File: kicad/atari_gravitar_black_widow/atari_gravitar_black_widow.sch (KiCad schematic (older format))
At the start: 2 parts

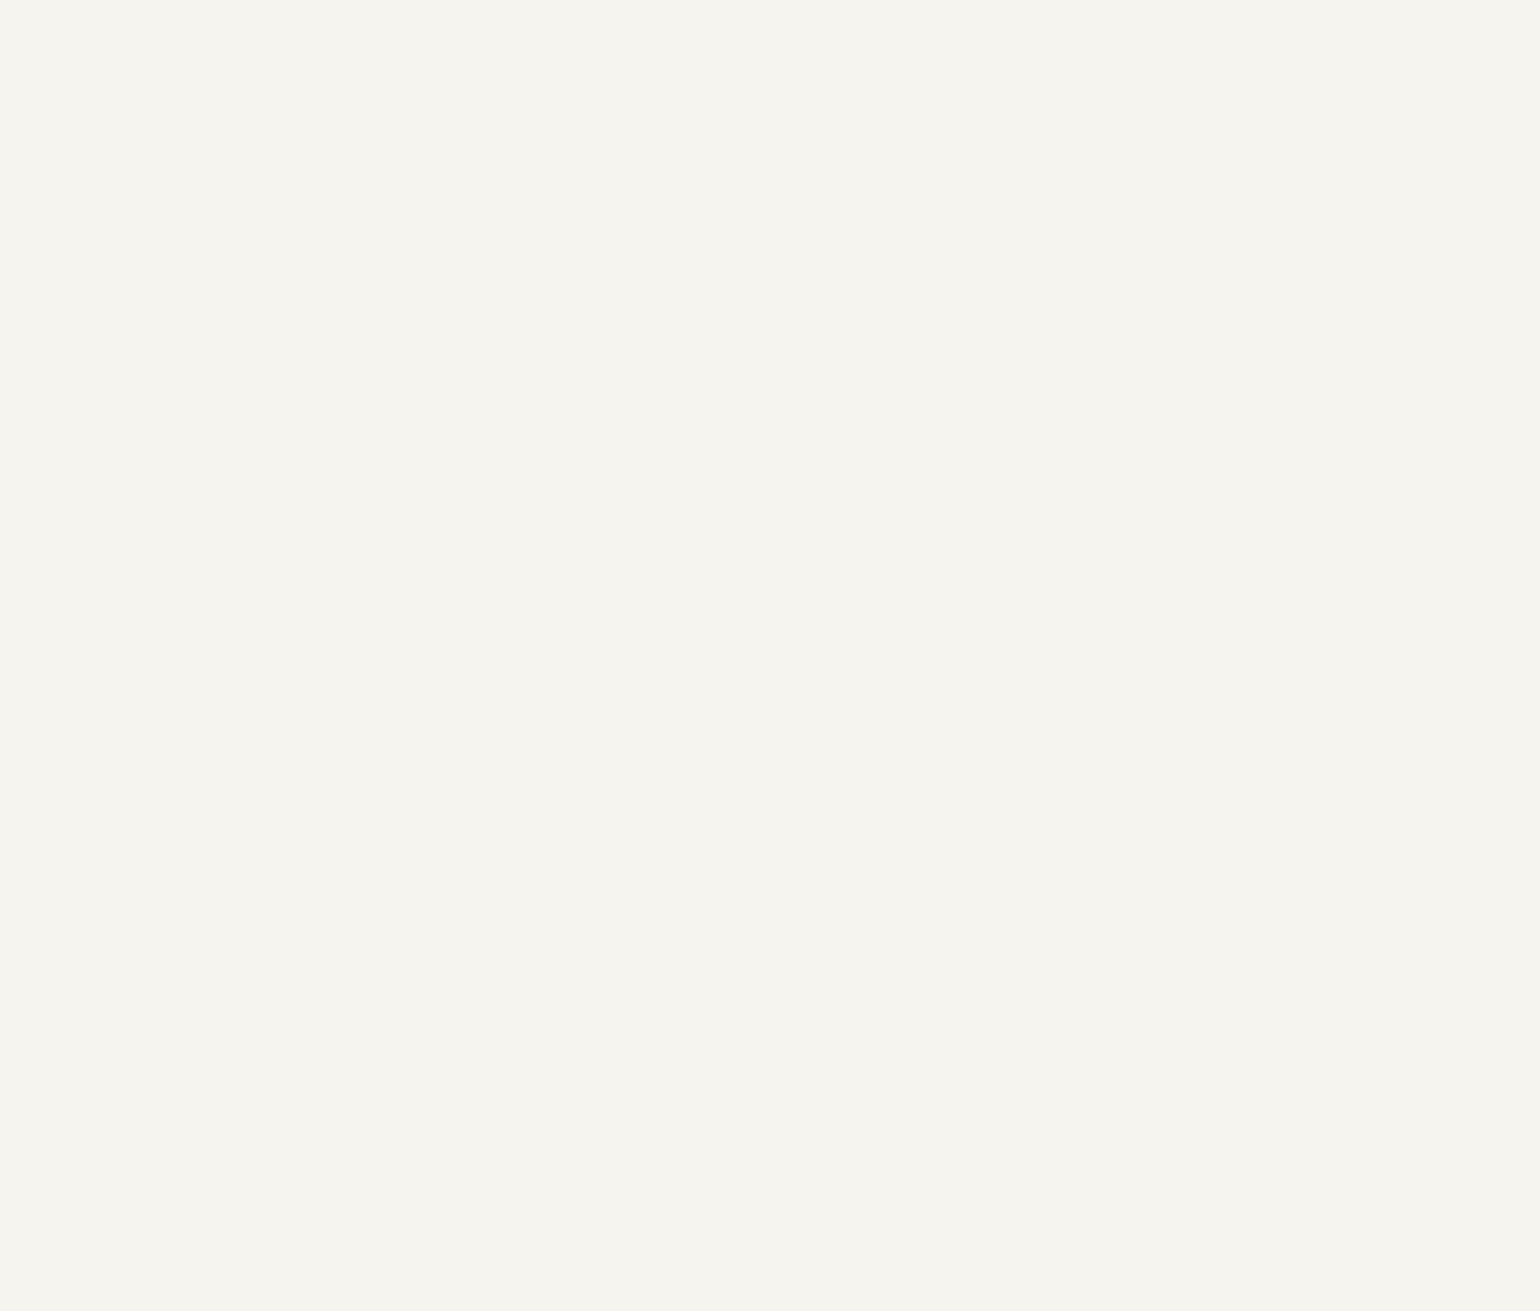
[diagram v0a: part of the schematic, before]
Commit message: First commit - AVG & VSM
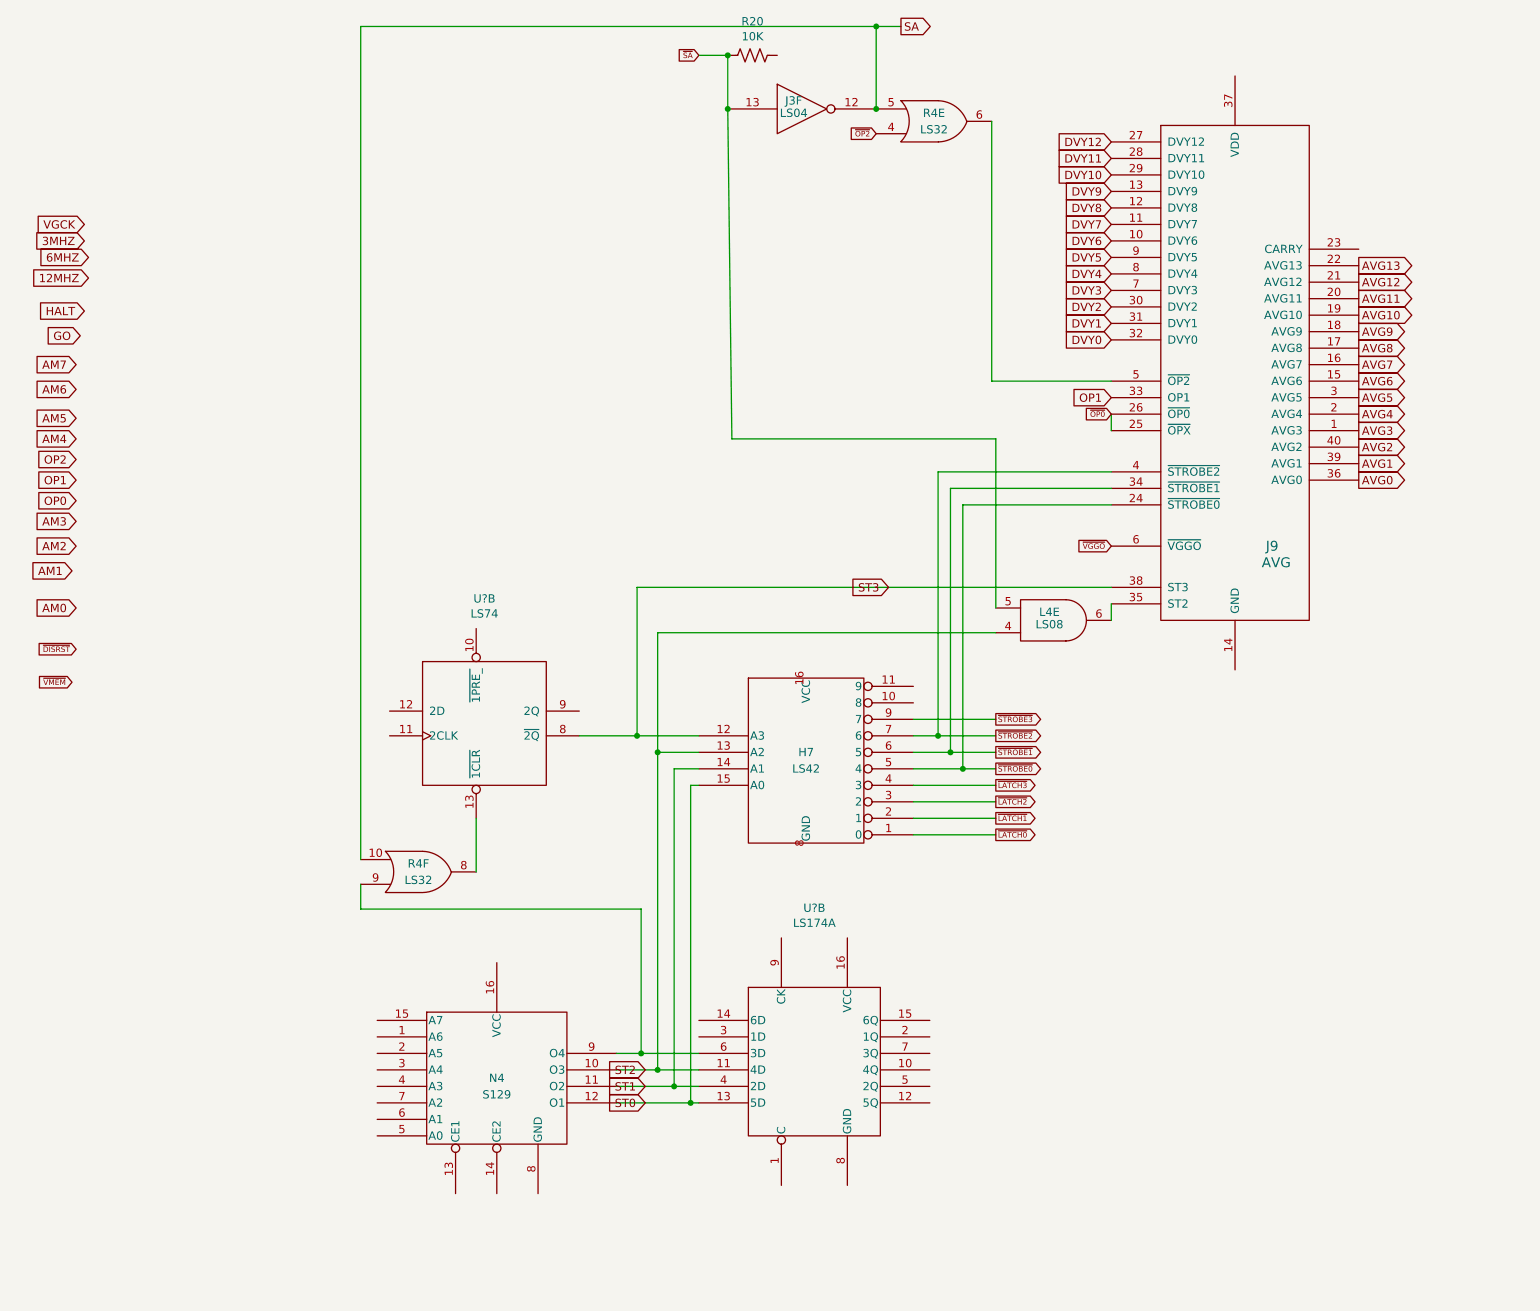
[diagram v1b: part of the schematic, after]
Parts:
- added H7: LS42, symbol Star_Wars_Vector_PCB:LS42
- added J3: LS04, symbol Star_Wars_Vector_PCB:LS04
- added J9: AVG, symbol Star_Wars_Vector_PCB:AVG
- added L4: LS08, symbol Star_Wars_Vector_PCB:LS08
- added N4: S129, symbol Star_Wars_Vector_PCB:S129
- added R20: 10K, symbol Device:R_US
- added R4: LS32, symbol Star_Wars_Vector_PCB:LS32
- added U?: LS74, symbol Star_Wars_Vector_PCB:LS74
- added U?: LS174A, symbol Star_Wars_Vector_PCB:LS174A
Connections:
- new net: J9.35 (ST2), L4.6
- new net: J9.5 (~OP2), R4.6
- new net: R4.8, U?.13 (~1CLR)
- new net: N4.9 (O4), R4.9, U?.6 (3D)
- new net AVG0: J9.36 (AVG0)
- new net AVG1: J9.39 (AVG1)
- new net AVG10: J9.19 (AVG10)
- new net AVG11: J9.20 (AVG11)
- new net AVG12: J9.21 (AVG12)
- new net AVG13: J9.22 (AVG13)
- new net AVG2: J9.40 (AVG2)
- new net AVG3: J9.1 (AVG3)
- new net AVG4: J9.2 (AVG4)
- new net AVG5: J9.3 (AVG5)
- new net AVG6: J9.15 (AVG6)
- new net AVG7: J9.16 (AVG7)
- new net AVG8: J9.17 (AVG8)
- new net AVG9: J9.18 (AVG9)
- new net DVY0: J9.32 (DVY0)
- new net DVY1: J9.31 (DVY1)
- new net DVY10: J9.29 (DVY10)
- new net DVY11: J9.28 (DVY11)
- new net DVY12: J9.27 (DVY12)
- new net DVY2: J9.30 (DVY2)
- new net DVY3: J9.7 (DVY3)
- new net DVY4: J9.8 (DVY4)
- new net DVY5: J9.9 (DVY5)
- new net DVY6: J9.10 (DVY6)
- new net DVY7: J9.11 (DVY7)
- new net DVY8: J9.12 (DVY8)
- new net DVY9: J9.13 (DVY9)
- new net OP1: J9.33 (OP1)
- new net SA: J3.12, R4.10, R4.5
- new net ST0: H7.15 (A0), N4.12 (O1), U?.13 (5D)
- new net ST1: H7.14 (A1), N4.11 (O2), U?.4 (2D)
- new net ST2: H7.13 (A2), L4.4, N4.10 (O3), U?.11 (4D)
- new net ST3: H7.12 (A3), J9.38 (ST3), U?.8 (~2Q)
- new net ~LATCH0: H7.1 (0)
- new net ~LATCH1: H7.2 (1)
- new net ~LATCH2: H7.3 (2)
- new net ~LATCH3: H7.4 (3)
- new net ~OP0: J9.25 (~OPX), J9.26 (~OP0)
- new net ~OP2: R4.4
- new net ~SA: J3.13, L4.5, R20.2
- new net ~STROBE0: H7.5 (4), J9.24 (~STROBE0)
- new net ~STROBE1: H7.6 (5), J9.34 (~STROBE1)
- new net ~STROBE2: H7.7 (6), J9.4 (~STROBE2)
- new net ~STROBE3: H7.9 (7)
- new net ~VGGO: J9.6 (~VGGO)

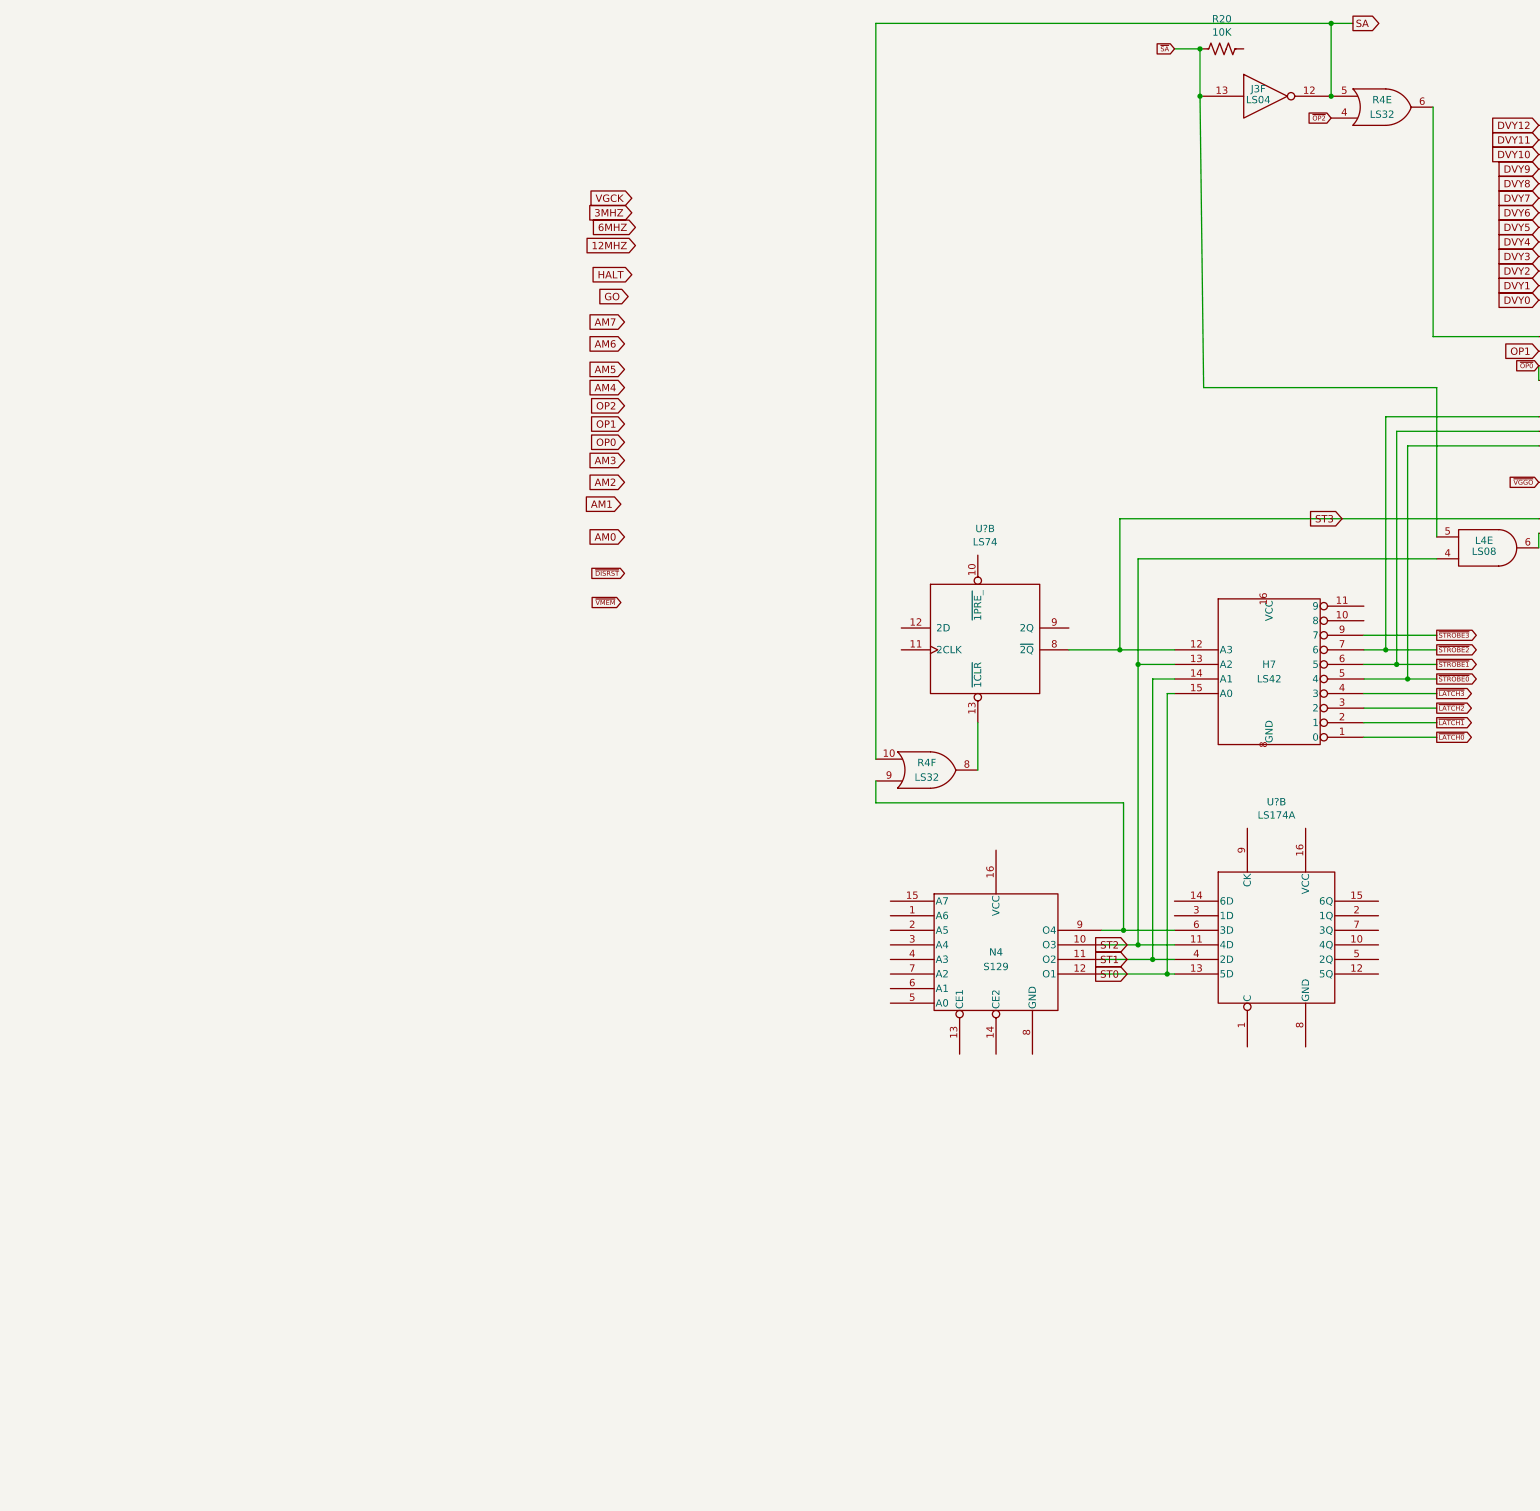
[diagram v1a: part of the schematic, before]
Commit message: 6B
More sheet 6B (but not all)
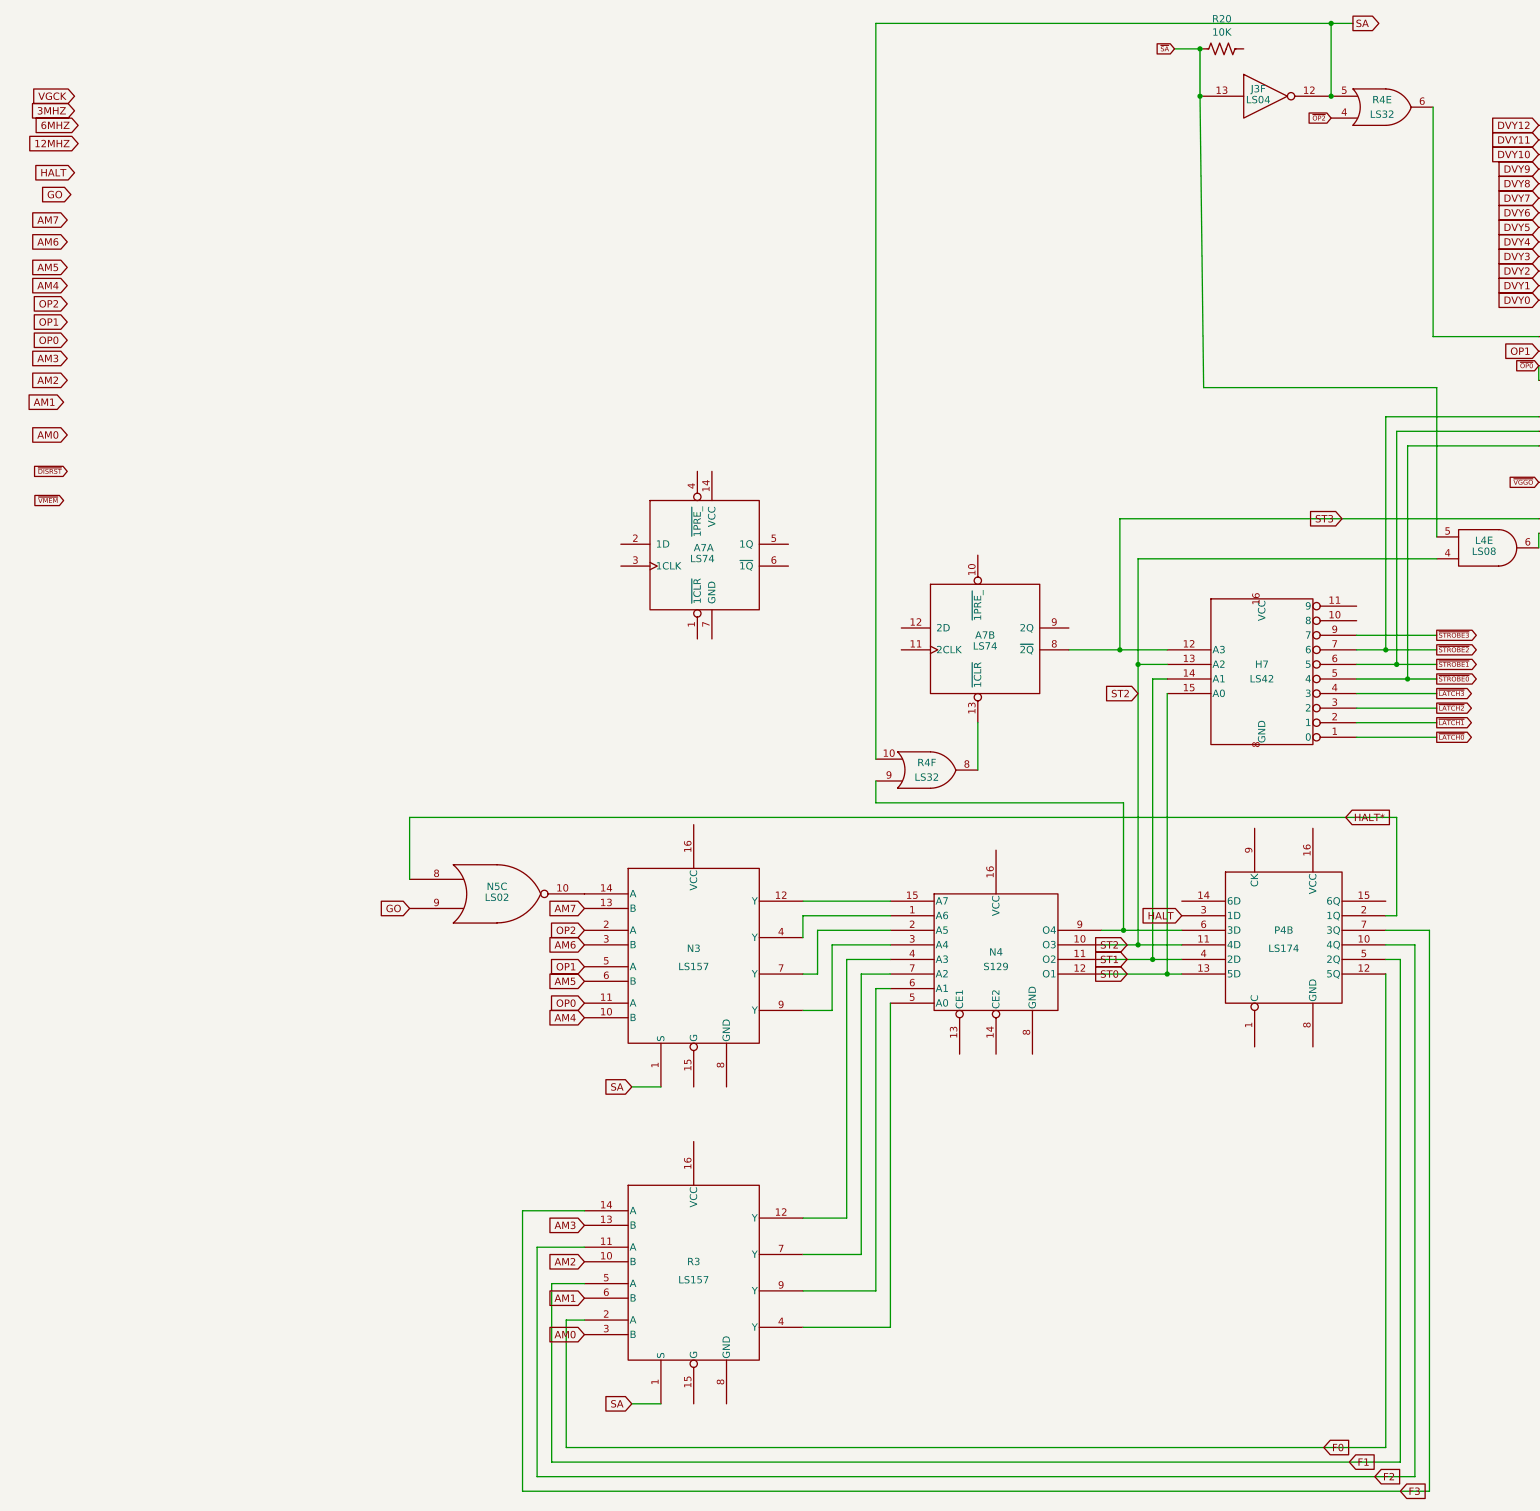
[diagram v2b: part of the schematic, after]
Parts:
- added unit 1 of A7
- added N3: LS157, symbol Star_Wars_Vector_PCB:LS157D
- added N5: LS02, symbol Star_Wars_Vector_PCB:LS02
- added R3: LS157, symbol Star_Wars_Vector_PCB:LS157C
- P4: renamed from U?; value LS174A -> LS174
- gave numbers to parts that had none: 1
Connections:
- net AM0: now also R3.3 (B)
- net AM1: now also R3.6 (B)
- net AM2: now also R3.10 (B)
- net AM3: now also R3.13 (B)
- net AM4: now also N3.10 (B)
- net AM5: now also N3.6 (B)
- net AM6: now also N3.3 (B)
- net AM7: now also N3.13 (B)
- net GO: now also N5.9
- net HALT: now also P4.3 (1D)
- net OP0: now also N3.11 (A)
- net OP1: now also N3.5 (A)
- net OP2: now also N3.2 (A)
- net SA: now also N3.1 (S), R3.1 (S)
- net F2: now reaches P4.10 (4Q)
- net F2: now also R3.11 (A)
- net F0: now reaches P4.12 (5Q)
- net F0: now also R3.2 (A)
- net HALT*: now reaches P4.2 (1Q)
- net HALT*: now also N5.8
- net F1: now reaches P4.5 (2Q)
- net F1: now also R3.5 (A)
- net F3: now reaches P4.7 (3Q)
- net F3: now also R3.14 (A)
- net at N4.1 (A6): now also N3.4 (Y)
- net at N4.15 (A7): now also N3.12 (Y)
- net at N4.2 (A5): now also N3.7 (Y)
- net at N4.3 (A4): now also N3.9 (Y)
- net at N4.4 (A3): now also R3.12 (Y)
- net at N4.5 (A0): now also R3.4 (Y)
- net at N4.6 (A1): now also R3.9 (Y)
- net at N4.7 (A2): now also R3.7 (Y)
- new net: N3.14 (A), N5.10
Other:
- moved on the sheet: H7, P4B
